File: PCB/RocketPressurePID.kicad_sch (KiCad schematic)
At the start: 47 parts, among them J1 TYPE-C 16PIN 2MD(073), J2 2x14 1.27mm SMD, J6 S5B-PH-SM4-TB(LF)(SN), Q4 IRLML2502TRPBF, SW1 TS-1002S-08026C, SW2 TS-1002S-08026C, U3 AMS1117-3.3, U4 M24C02-FMN, U5 STM32G030C8Tx, Y2 8 MHz

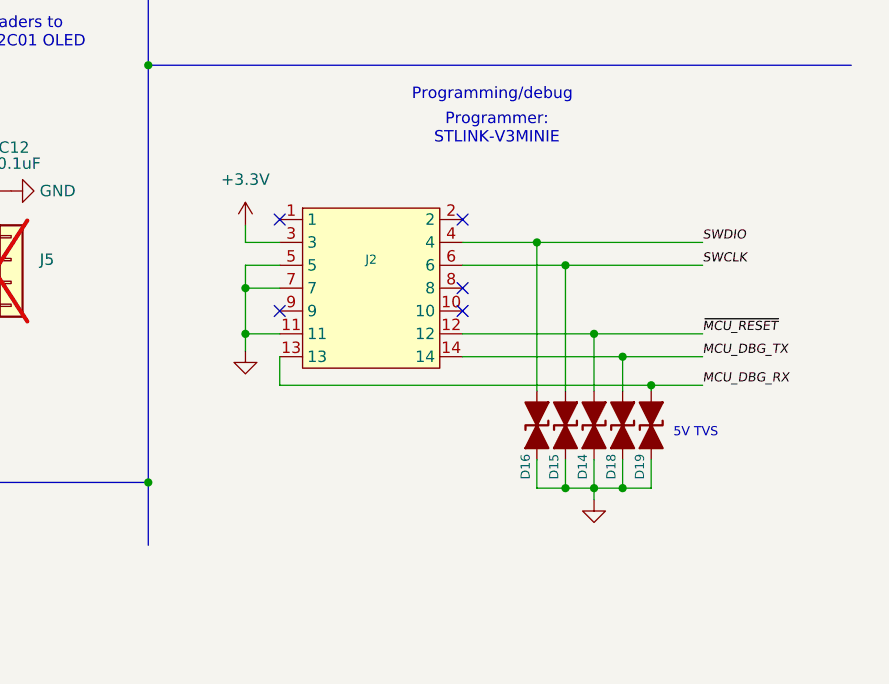
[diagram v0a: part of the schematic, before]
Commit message: WIP
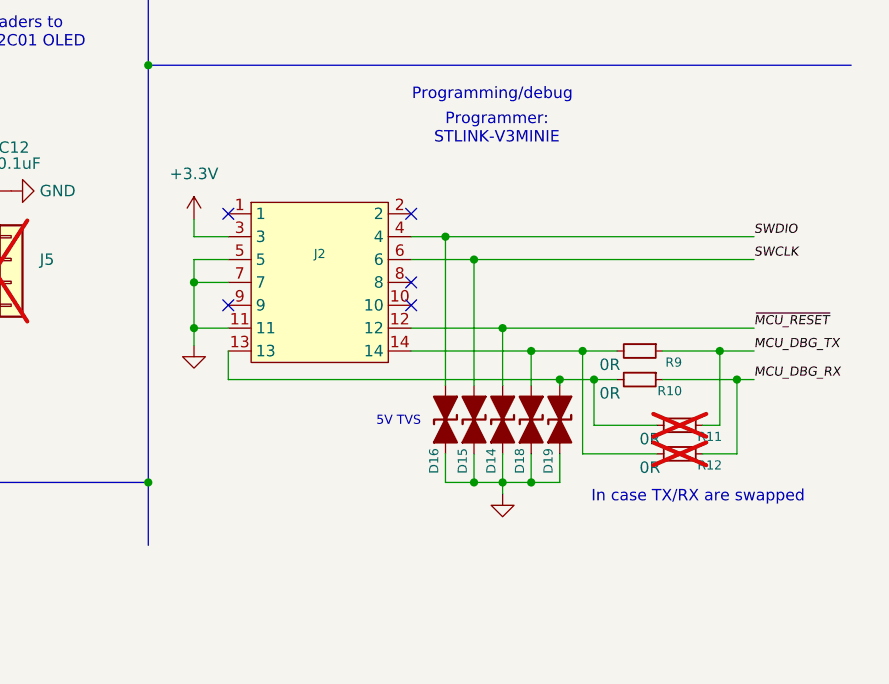
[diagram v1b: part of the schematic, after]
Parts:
- added R10, R11, R12, R9: 0R, Resistor_SMD:R_0603_1608Metric, symbol Device:R_Small
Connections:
- net MCU_DBG_RX: now also R10.1, R12.1; no longer D19.1 (A1), J2.13
- net MCU_DBG_TX: now also R11.1, R9.1; no longer D18.1 (A1), J2.14
- new net: D19.1 (A1), J2.13, R10.2, R11.2
- new net: D18.1 (A1), J2.14, R12.2, R9.2
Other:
- note added: "In case TX/RX are swapped"
- moved on the sheet: D14, D15, D16, D18, D19, J2
